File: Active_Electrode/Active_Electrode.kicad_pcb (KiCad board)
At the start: 2 copper layers, 14 parts, among them J1 Conn_01x02, J2 Conn_01x09, U1 ADG442BNZ, U2 LF412

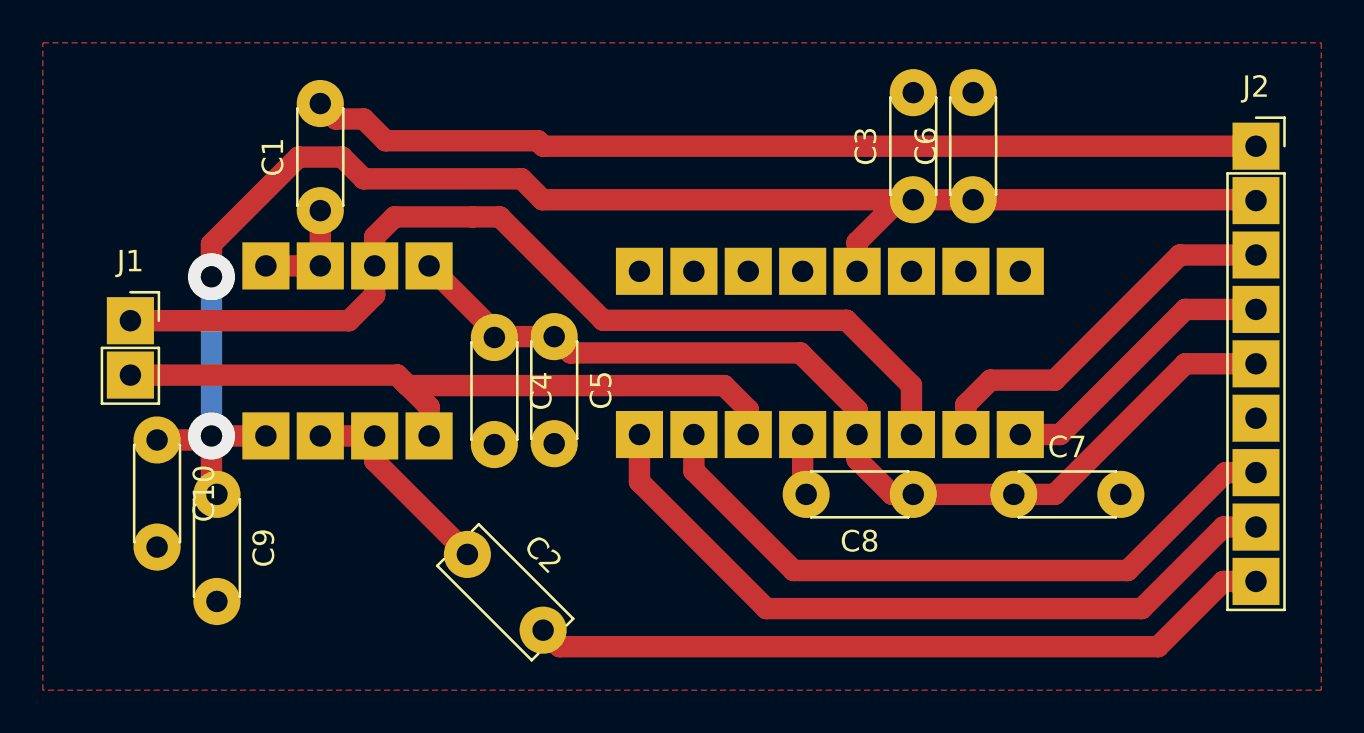
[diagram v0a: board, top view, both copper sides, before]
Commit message: Active Electrode
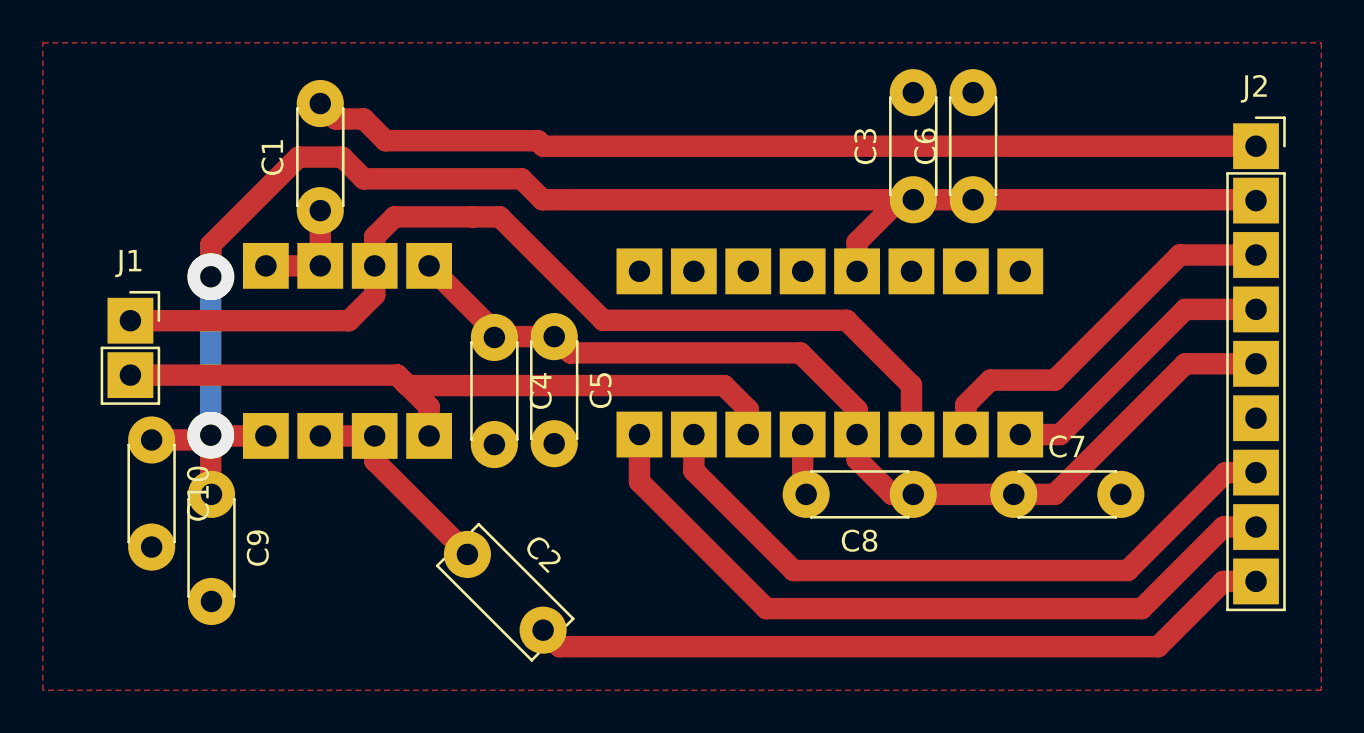
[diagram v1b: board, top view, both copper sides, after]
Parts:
- moved C9 0.25 mm to (7.87, 21.1)
- moved C10 0.25 mm to (5.08, 18.5)
